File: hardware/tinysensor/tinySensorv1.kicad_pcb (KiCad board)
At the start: 2 copper layers, 97.9 x 63.8 mm, 40 parts, among them J1 RADIO, J10 CR2032 socket, J11 AAA socket, J12 AA Socket, J13 RAW IN, J2 DCDC converter, J3 I2C Sensor (BME/BMP 280), J4 Digital out, J5 OneWire sensor, J6 ISP, J7 Analog sensor, J8 EXT. INT0, SW1 RESET, U1 ATtiny84A-PU

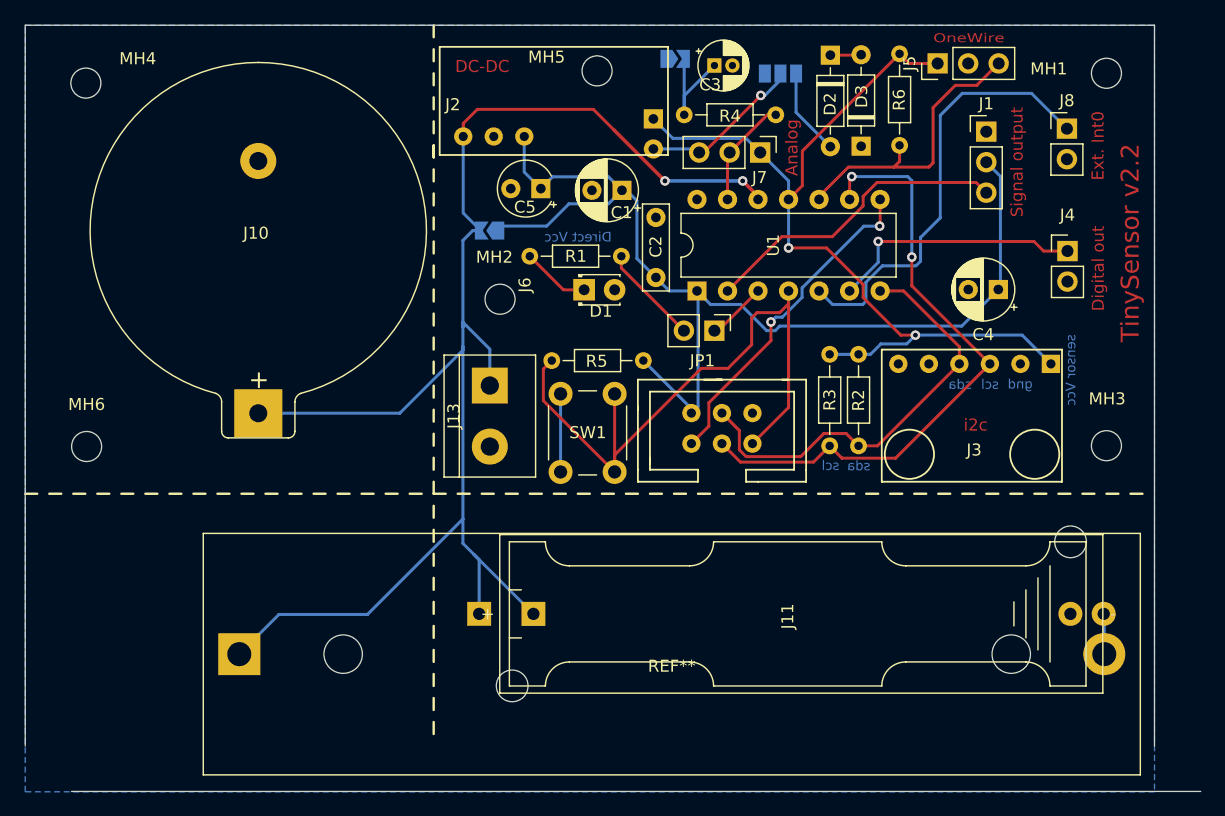
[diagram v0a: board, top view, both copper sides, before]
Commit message: hardware: Update of Kikad design, new batch expected
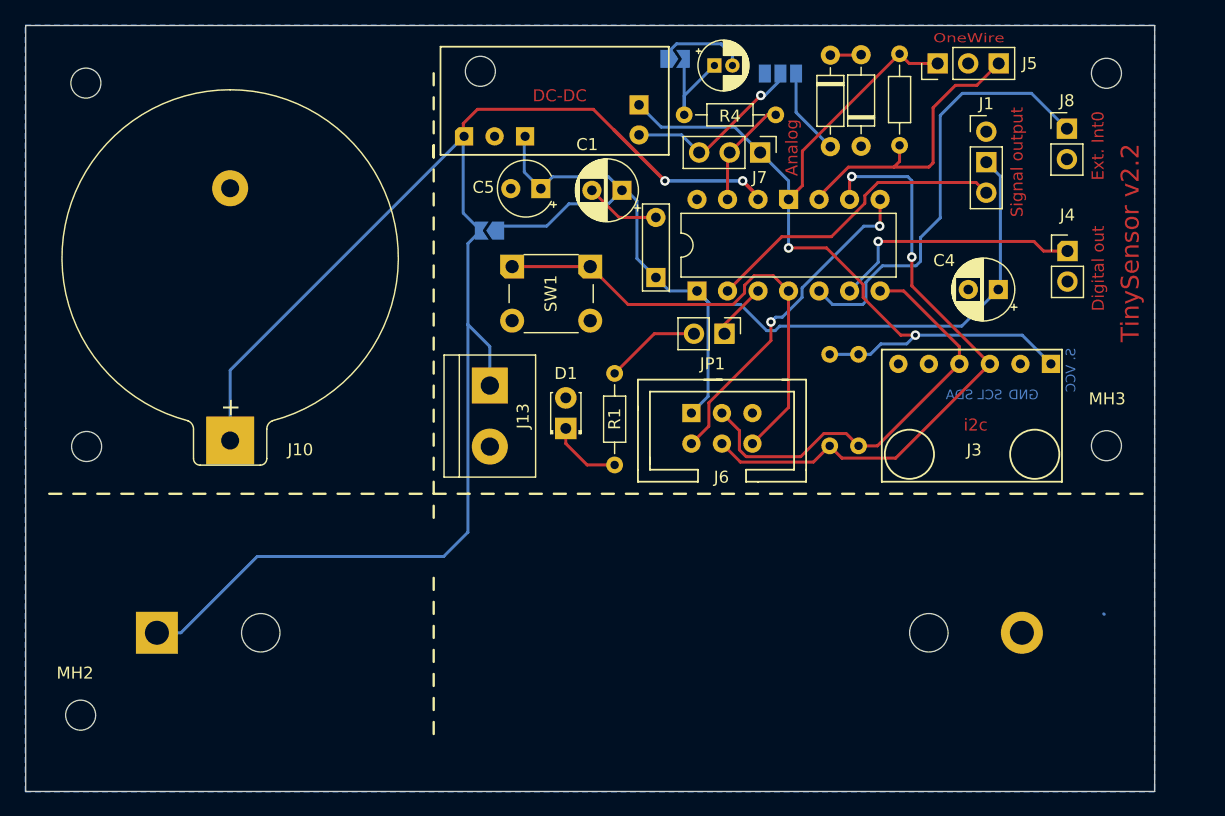
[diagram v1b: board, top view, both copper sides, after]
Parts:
- removed J11: AAA socket, Battery:BatteryHolder_Keystone_2466_1xAAA
- removed J12: AA Socket, Battery:BatteryHolder_Keystone_2460_1xAA
- removed R5: 10k, Resistor_THT:R_Axial_DIN0204_L3.6mm_D1.6mm_P7.62mm_Horizontal
- removed REF**: BatteryHolder_MPD_BH-18650-PC2, Battery:BatteryHolder_MPD_BH-18650-PC2
- added 18650: BatteryHolder_MPD_BH-18650-PC2, Battery:BatteryHolder_MPD_BH-18650-PC2, B.Cu at (124.0, 98.6)
- R2, R3: moved to B.Cu
- moved MH2 49.2 mm to (117.6, 105.4)
- moved R1 18.8 mm to (162.1, 84.6), turned to 90 degrees
- moved SW1 13.6 mm to (153.5, 68.1), turned to 0 degrees
- moved D1 11.6 mm to (158.0, 81.6), turned to 90 degrees
- moved MH5 9.71 mm to (150.9, 51.8)
- moved J10 3.26 mm to (130.1, 82.6)
- moved C6 1.67 mm to (164.1, 54.6)
- moved JP1 0.88 mm to (171.2, 73.7)
- moved J2 0.07 mm to (147.6, 58.8)
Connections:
- D1 pad 1: (no net) -> Net-(D1-K)
- R1 pad 1: Net-(D1-Pad1) -> Net-(D1-K)
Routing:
- net /RESET: track 54.9 -> 40.2 mm
- net Net-(D1-K): track 0.00 -> 6.07 mm
- net Net-(D1-Pad1): track 5.68 -> 0.00 mm
- net VCC: track 92.2 -> 87.3 mm
- net +BATT: track 127.7 -> 131.9 mm
- net GND: track 9.87 -> 13.8 mm
- net Net-(J7-Pin_3): track 14.5 -> 16.1 mm
- net /SENSOR_VCC: track 72.7 -> 74.4 mm
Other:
- board size 97.9 x 63.8 mm -> 94 x 63.8 mm
- board text added: "GND"
- board text added: "S. VCC"
- board text added: "SCL"
- board text added: "SDA"
- board text removed: "Direct Vcc"
- board text removed: "gnd"
- board text removed: "scl"
- board text removed: "sda"
- board text removed: "sensor Vcc"
